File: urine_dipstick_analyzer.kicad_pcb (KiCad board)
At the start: 2 copper layers, 50 x 30 mm, 28 parts, among them J1 BAT, J2 9V_OUT, J3 3V3_OUT, J4 I2C_BUS, J5 MOTOR_PWR, U1 MCP73833, U1a USB-C-BO, U4 MAX17048

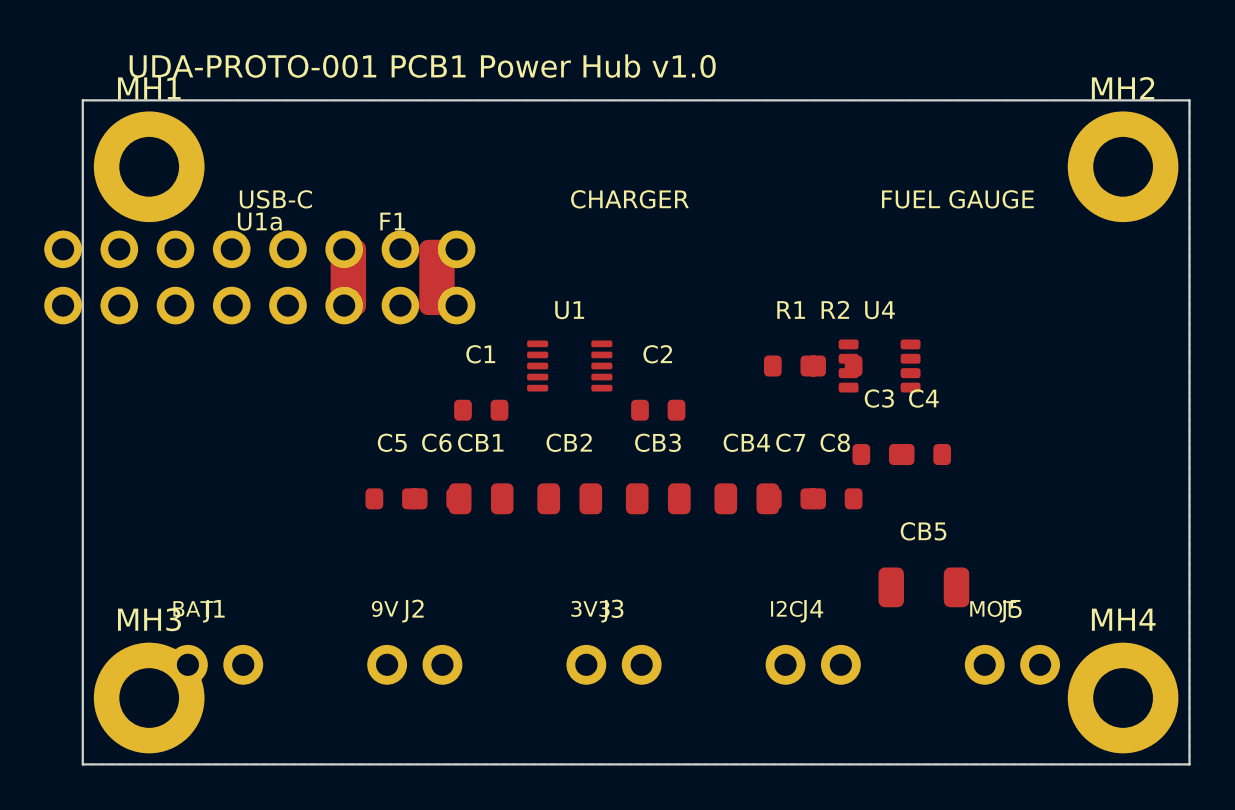
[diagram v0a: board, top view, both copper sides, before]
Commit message: Route PCB, add README+LICENSE, verify firmware build
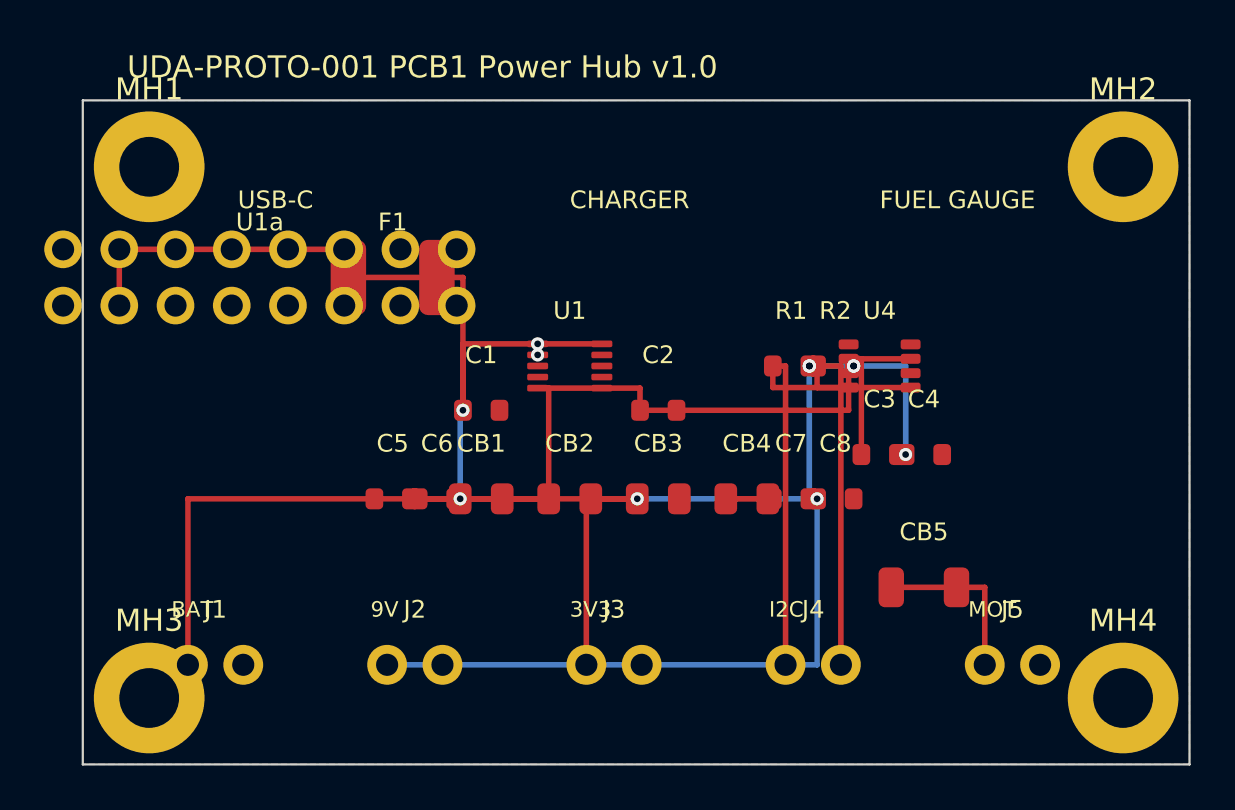
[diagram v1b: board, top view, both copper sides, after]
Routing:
- net VBAT: track 0.00 -> 54.4 mm
- net +3V3: track 0.00 -> 41.8 mm, vias 0 -> 6
- net VBUS: track 0.00 -> 38.7 mm, vias 0 -> 2
- net +9V: track 0.00 -> 26.9 mm, vias 0 -> 1
- net SCL: track 0.00 -> 19.8 mm
- net SDA: track 0.00 -> 18.5 mm
- net VMOT: track 0.00 -> 7.73 mm
- net +5V: track 0.00 -> 2.12 mm
- net CHRG_STAT: track 0.00 -> 0.50 mm, vias 0 -> 2
